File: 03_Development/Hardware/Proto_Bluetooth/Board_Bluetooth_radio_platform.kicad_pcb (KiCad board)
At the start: 2 copper layers, 218 x 124 mm, 103 parts, among them J1 Conn_01x02, J10 Conn_01x03, J11 HMI_rotaryEncoder_1, J12 HMI_rotaryEncoder_1, J13 Conn_01x08_epaper, J14 Conn_01x03_fmModule_audioOutp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, J15 Conn_01x02_classD_SD, J19 Conn_01x02_rn52_usb, J2 Conn_01x08, J20 Conn_01x05_toClassD, J3 BT_RN52_connector_left, J4 Conn_01x02, J5 BT_RN52_connector_right, J6 FM_interface, J7 BT_debug_connector, J8 BT_extension_connector, J9 SYS_debug_connector, SW1 SW_Push, U1 LM317_TO-220, U3 TPA6112A2DGQ, U4 TS5A2234

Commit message: [HDW_43] FIX PCB edges for mechanical fit in Radio
Left side is not fully filled as we need a space for Bluetooth
antenna's
Space for loudspeaker had to be increased
Right upper size had to be reduced of a couple of cm
Left spaces had some space avaialble which is now used
Ready for button resync and replace of components
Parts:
- moved C2 59.9 mm to (221.2, 47.3)
- moved C3 59.9 mm to (226.5, 49.7)
- moved D1 59.9 mm to (244.6, 39.1)
- moved J1 59.9 mm to (273.8, 45.1)
- moved J11 59.9 mm to (190.5, 48.3)
- moved J15 59.9 mm to (136.3, 93.2)
- moved J3 59.9 mm to (132.6, 101.5)
- moved J_I1 59.9 mm to (272.7, 33.4)
- moved J_III1 59.9 mm to (231.4, 33.4)
- moved J_VIII1 59.9 mm to (128.2, 33.4)
- moved J_pwrLed1 59.9 mm to (230.3, 57.1)
- moved R10 59.9 mm to (226.5, 55.6)
- moved R28 59.9 mm to (171.0, 64.2)
- moved R31 59.9 mm to (194.8, 38.6)
- moved R32 59.9 mm to (194.8, 36.0)
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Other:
- board size 218 x 124 mm -> 220.5 x 124 mm

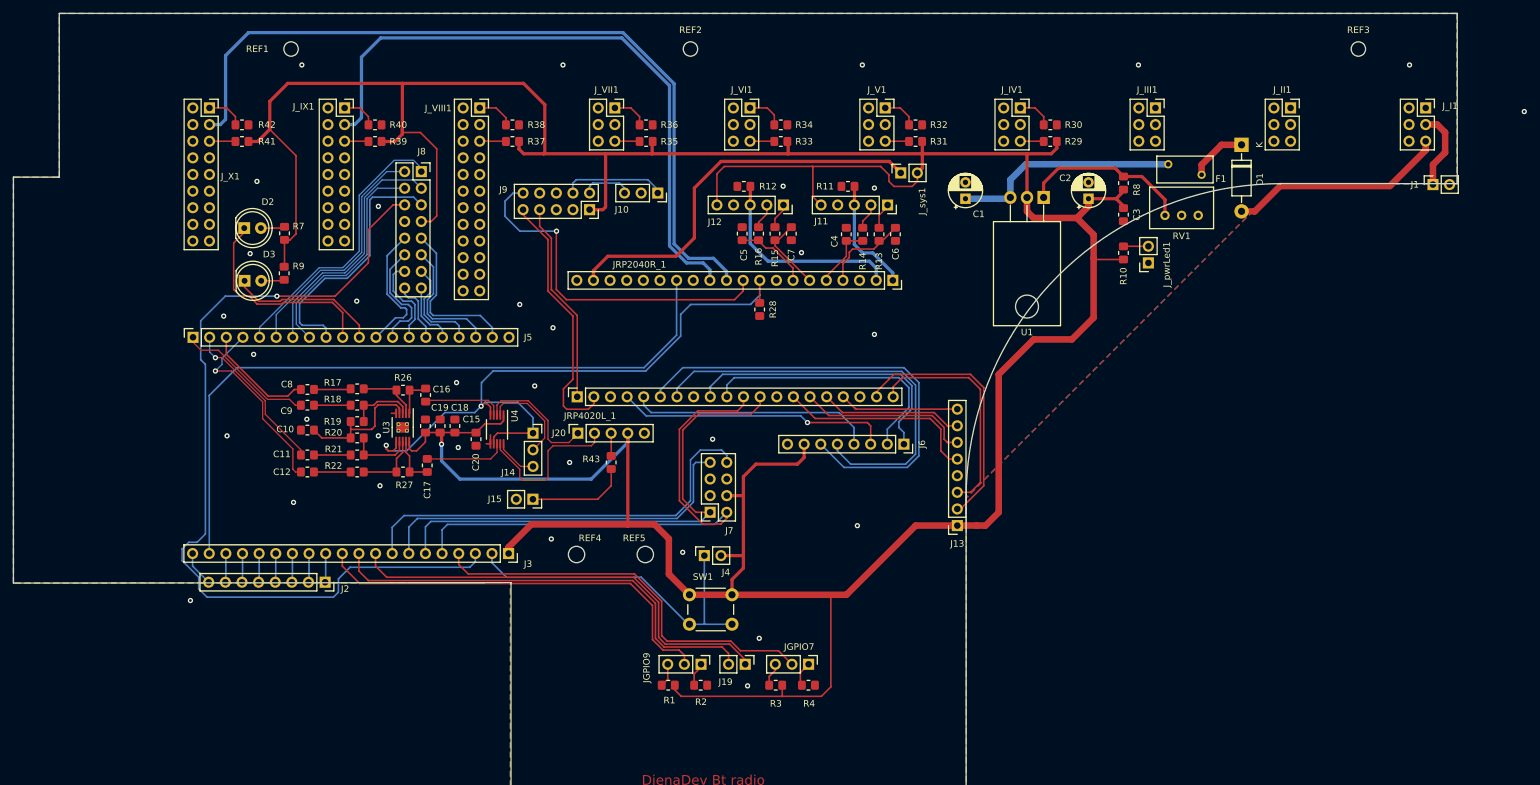
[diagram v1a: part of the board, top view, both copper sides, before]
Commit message: [HDW_44][HDW_42][HDW_50] FIX all of those topics
Move mounting hole to their correct place
Push buttons are good and works as expected
Place of specific headers for push-buttons is now corrected
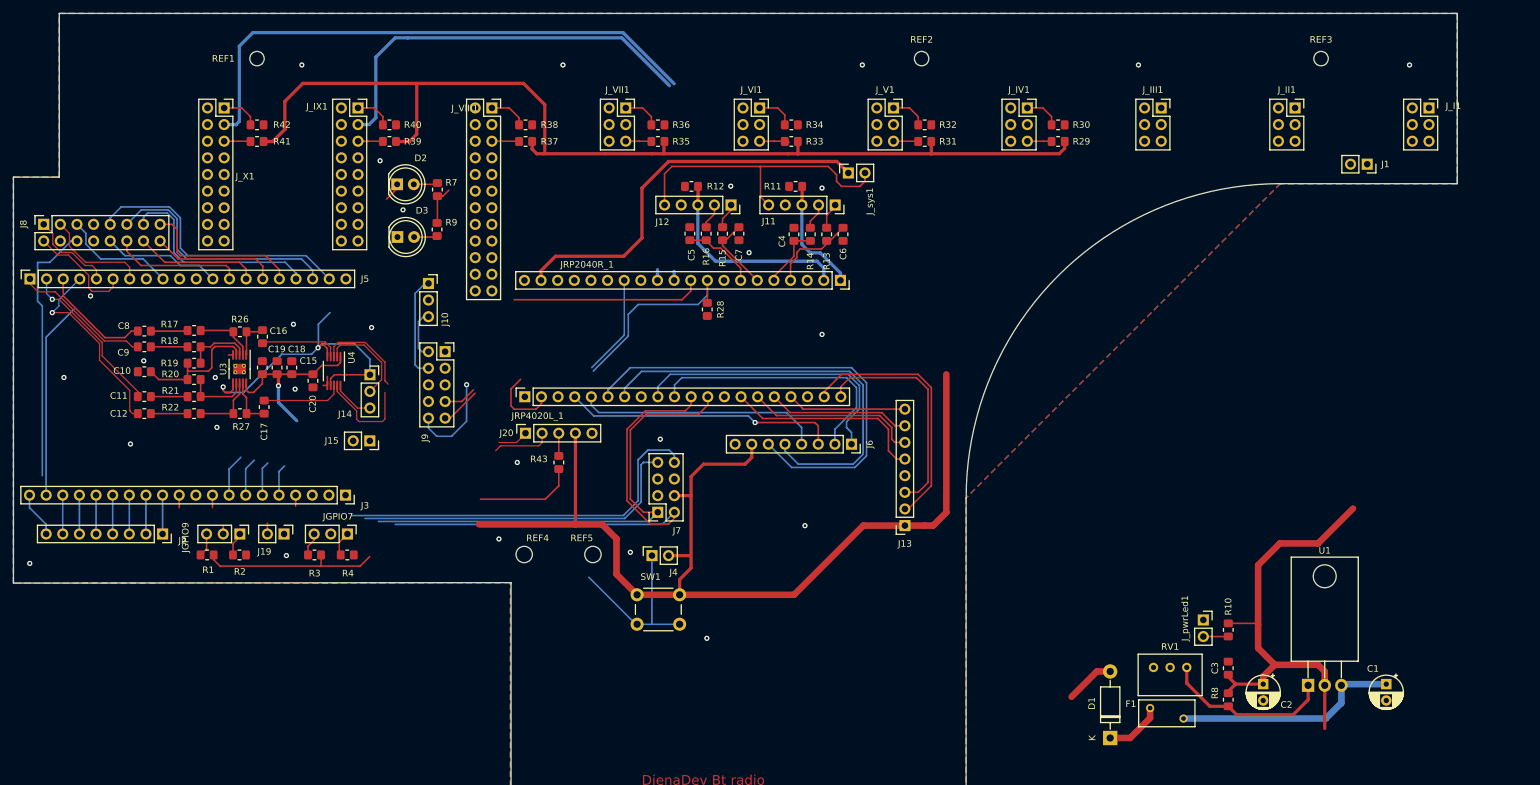
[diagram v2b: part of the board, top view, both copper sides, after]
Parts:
- moved C1 98.1 mm to (266.7, 121.4), turned to -90 degrees
- moved D1 92.8 mm to (224.5, 129.7), turned to 90 degrees
- moved U1 84.8 mm to (254.7, 121.6), turned to 0 degrees
- moved F1 81.8 mm to (230.6, 125.1), turned to 0 degrees
- moved R8 80.5 mm to (242.5, 123.8), turned to -90 degrees
- moved C2 78.8 mm to (247.9, 121.4), turned to -90 degrees
- moved R2 73.2 mm to (91.5, 101.7)
- moved J19 73.2 mm to (98.3, 98.5)
- moved JGPIO7 73.2 mm to (108.0, 98.5)
- moved JGPIO9 73.2 mm to (91.6, 98.5)
- moved R1 73.2 mm to (86.6, 101.7)
- moved R3 73.2 mm to (103.0, 101.7)
- moved R4 73.2 mm to (108.0, 101.7)
- moved C3 71.1 mm to (242.5, 119.0), turned to 90 degrees
- moved RV1 69.1 mm to (236.2, 118.9), turned to 0 degrees
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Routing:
- net +3V3: track 594.1 -> 490.2 mm
- net BT_GPIO6: track 133.4 -> 40.2 mm, vias 1 -> 0
- net Net-(J19-Pad2): track 69.1 -> 1.64 mm
- net Net-(J19-Pad1): track 68.1 -> 2.62 mm
- net BT_GPIO2: track 107.7 -> 45.5 mm
- net BT_GPIO9: track 64.2 -> 3.28 mm
- net BT_GPIO7: track 62.0 -> 1.67 mm
- net sys_button_a: track 121.3 -> 85.9 mm
- net BT_MIC_L+: track 34.9 -> 0.00 mm
- net sys_button_b: track 97.3 -> 63.0 mm
- net BT_MIC_R-: track 42.8 -> 13.3 mm
- net BT_LED_0: track 32.1 -> 2.94 mm
- net DBG_UART_RX: track 31.0 -> 5.05 mm
- net sys_onoff_o: track 33.4 -> 7.50 mm
- net BT_PWREN: track 52.6 -> 27.5 mm
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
